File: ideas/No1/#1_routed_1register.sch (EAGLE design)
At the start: 17 parts, among them IC1 ULN2803, IC2 ULN2803, IC3 TD620831A, IC4 TD620831A, U1 SN74HC595N, U2 SN74HC595N, U3 SN74HC595N, U4 SN74HC595N

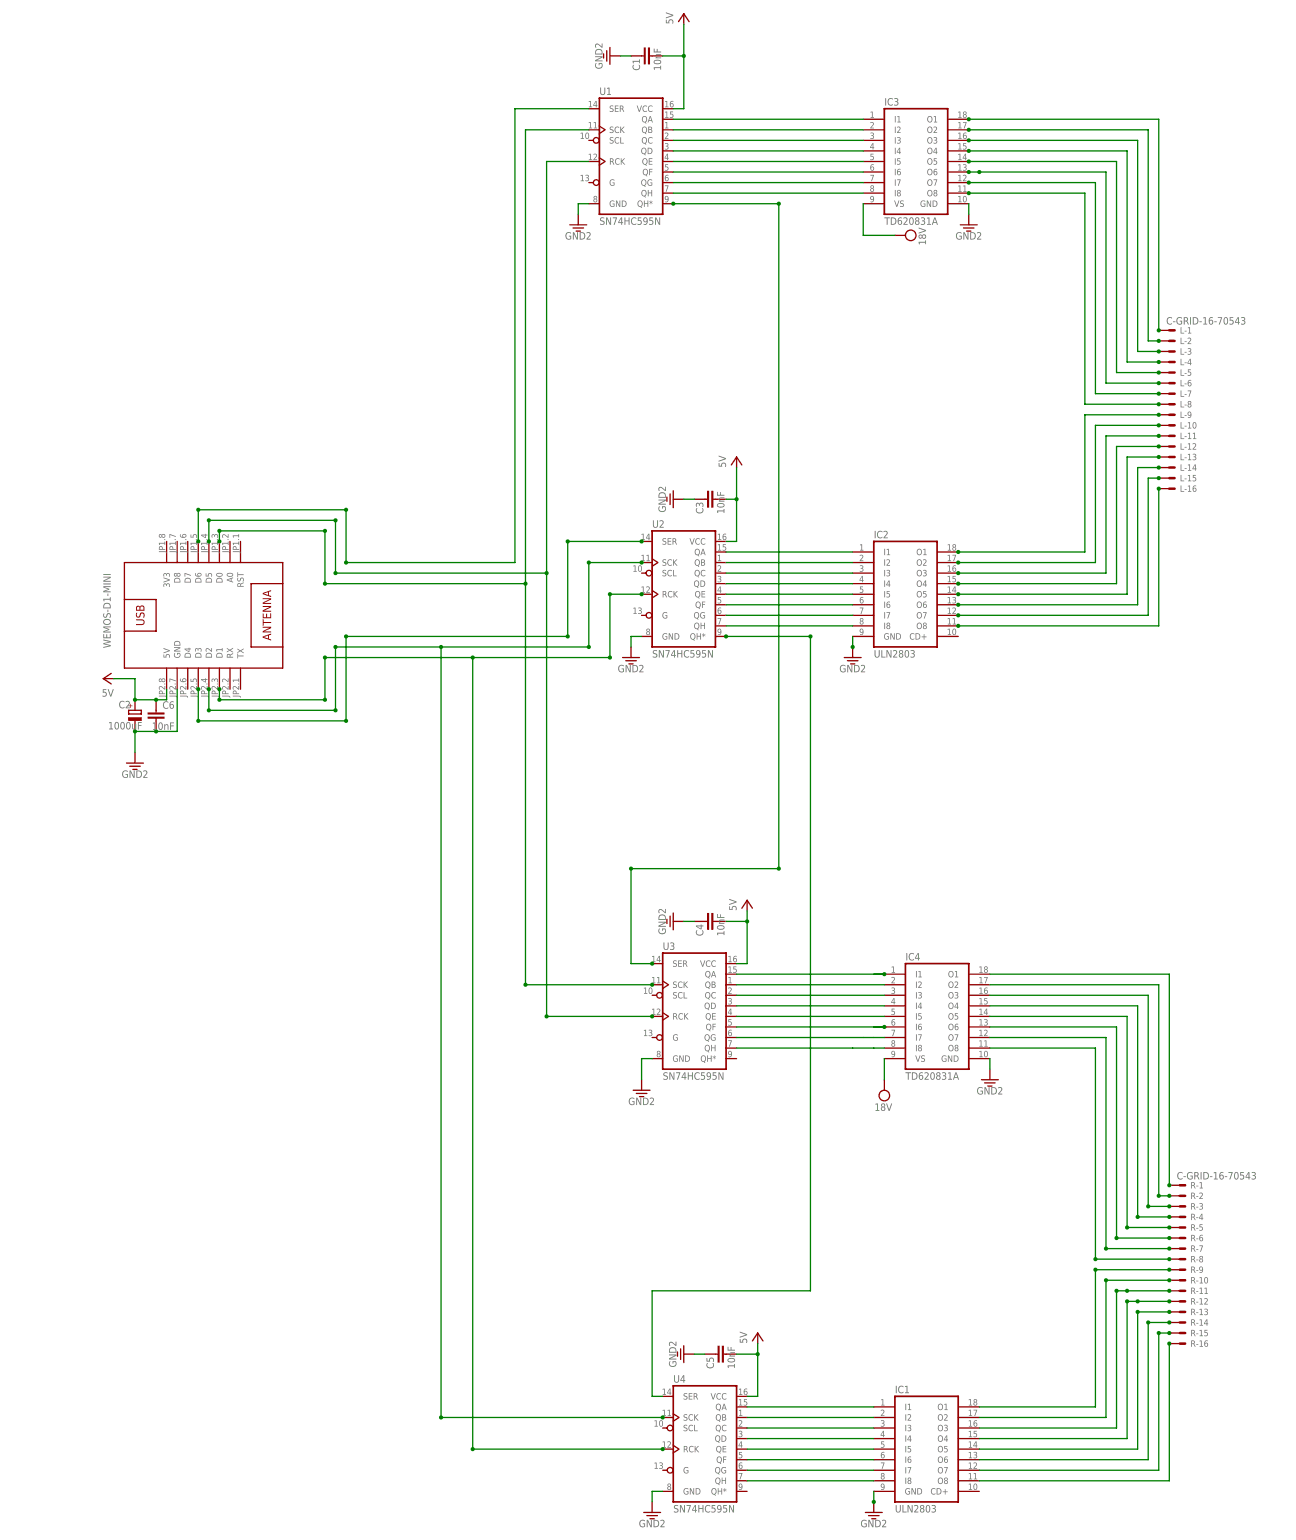
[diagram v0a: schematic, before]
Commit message: 1_route_1register.sch
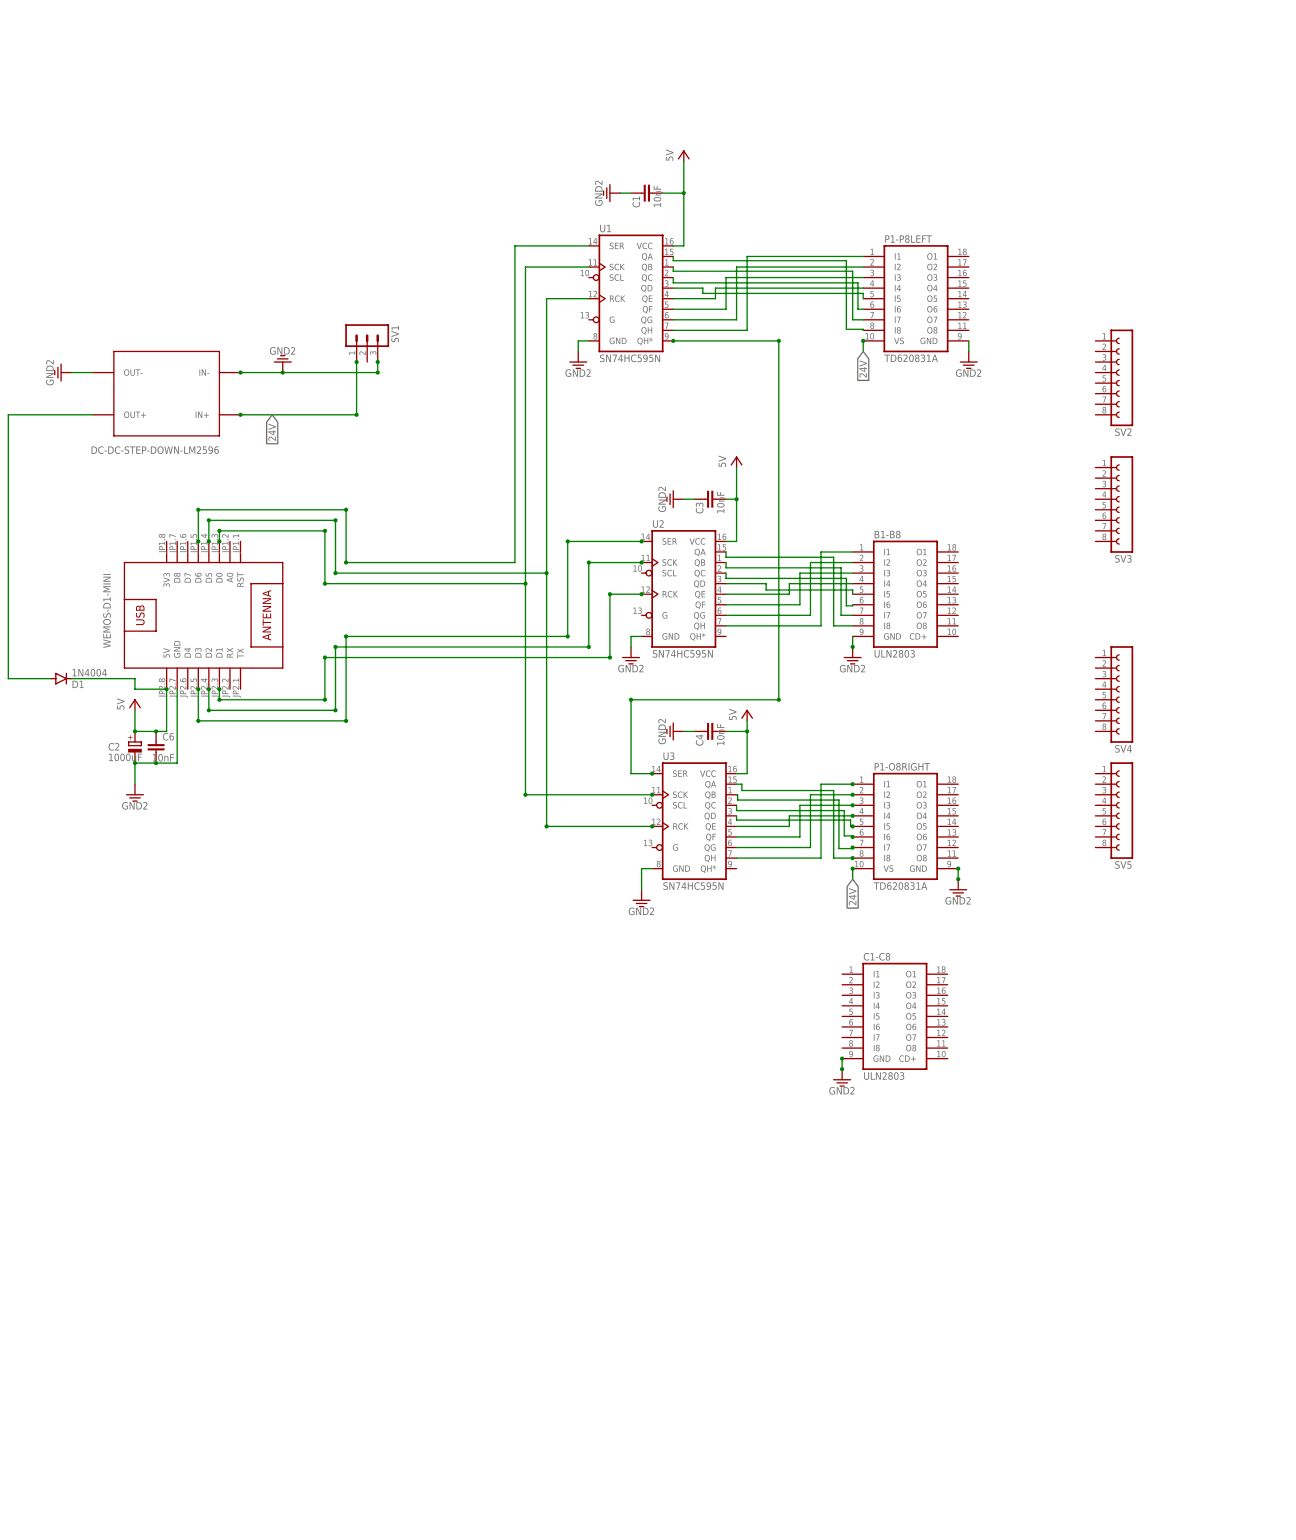
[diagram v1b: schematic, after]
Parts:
- removed C5: 10nF, resistor:C-EU025-025X050
- removed IC1: ULN2803, uln-udn:ULN2803A
- removed IC3, IC4: TD620831A, td62083-dil:TD620831A
- removed L, R: C-GRID-16-70543, con-molex:C-GRID-16-70543
- removed U4: SN74HC595N, SparkFun-IC-Logic:74HC595N
- added C1-C8: ULN2803, uln-udn:ULN2803A
- added D1: 1N4004, diode:1N4004
- added P1-O8RIGHT, P1-P8LEFT: TD620831A, td62083-dil:TD620831A
- added SV1: (no value), con-lstb:MA03-1
- added SV2, SV3, SV4, SV5: (no value), con-lsta:FE08-1
- added U$2: DC-DC-STEP-DOWN-LM2596, diy-modules_lm2596:DC-DC-STEP-DOWN-LM2596
- renumbered IC2 to B1-B8
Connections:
- removed net N$10: IC3.O2, L-2.S
- removed net N$11: IC3.O3, L-3.S
- removed net N$12: IC3.O4, L-4.S
- removed net N$13: IC3.O5, L-5.S
- removed net N$14: IC3.O6, L-6.S
- removed net N$15: IC3.O7, L-7.S
- removed net N$16: IC3.O8, L-8.S
- removed net N$17: B1-B8.O8, L-16.S
- removed net N$18: B1-B8.O7, L-15.S
- removed net N$19: B1-B8.O6, L-14.S
- removed net N$20: B1-B8.O5, L-13.S
- removed net N$21: B1-B8.O4, L-12.S
- removed net N$22: B1-B8.O3, L-11.S
- removed net N$23: B1-B8.O2, L-10.S
- removed net N$24: B1-B8.O1, L-9.S
- removed net N$26: IC4.O2, R-2.S
- removed net N$28: IC4.O4, R-4.S
- removed net N$30: IC4.O6, R-6.S
- removed net N$33: IC4.O8, R-8.S
- removed net N$35: IC4.I8, U3.QH
- removed net N$39: IC1.O8, R-16.S
- removed net N$40: IC1.O7, R-15.S
- removed net N$49: IC1.O6, R-14.S
- removed net N$50: IC1.O5, R-13.S
- removed net N$51: IC1.O4, R-12.S
- removed net N$52: IC1.O3, R-11.S
- removed net N$53: IC1.O2, R-10.S
- removed net N$54: IC1.O1, R-9.S
- removed net N$57: IC4.O1, R-1.S
- removed net N$59: IC4.O3, R-3.S
- removed net N$61: IC4.O5, R-5.S
- removed net N$63: IC4.O7, R-7.S
- removed net N$73: IC4.I2, U3.QB
- removed net N$74: IC4.I3, U3.QC
- removed net N$75: IC4.I4, U3.QD
- removed net N$76: IC4.I5, U3.QE
- removed net N$77: U2.QH*, U4.SER
- removed net N$78: IC4.I7, U3.QG
- removed net N$83: IC1.I1, U4.QA
- removed net N$84: IC1.I2, U4.QB
- removed net N$85: IC1.I3, U4.QC
- removed net N$86: IC1.I4, U4.QD
- removed net N$87: IC1.I5, U4.QE
- removed net N$88: IC1.I6, U4.QF
- removed net N$89: IC1.I7, U4.QG
- removed net N$9: IC3.O1, L-1.S
- removed net N$90: IC1.I8, U4.QH
- new net 24V: P1-O8RIGHT.VS, P1-P8LEFT.VS, SV1.1, U$2.IN+
- new net GND: B1-B8.GND, C1-C8.GND, C1.1, C2.-, C3.1, C4.1, C6.2, P1-O8RIGHT.GND, P1-P8LEFT.GND, U$1.GND, U1.GND, U2.GND, U3.GND
- new net N$25: P1-P8LEFT.I1, U1.QH
- new net N$27: P1-P8LEFT.I2, U1.QG
- new net N$29: P1-P8LEFT.I3, U1.QF
- new net N$32: P1-P8LEFT.I5, U1.QD
- new net N$55: P1-O8RIGHT.I7, U3.QB
- new net N$56: P1-O8RIGHT.I8, U3.QA
- new net N$69: D1.A, U$2.OUT+
- net 3.3V: now also SV1.3, U$2.IN-, U$2.OUT-; no longer B1-B8.GND, C1.1, C2.-, C3.1, C4.1, C5.1, C6.2, IC1.GND, IC3.GND, IC4.GND, U$1.GND, U1.GND, U2.GND, U3.GND, U4.GND
- net N$1: now also U2.QH; no longer U2.QA
- net N$2: now also U2.QG; no longer U2.QB
- net N$3: now also U2.QF; no longer U2.QC
- net N$31: now also P1-P8LEFT.I4, U1.QE; no longer IC3.I8, U1.QH
- net N$38: no longer U4.RCK
- net N$4: now also U2.QE; no longer U2.QD
- net N$41: now also P1-P8LEFT.I6, U1.QC; no longer IC3.I1, U1.QA
- net N$42: now also P1-P8LEFT.I7; no longer IC3.I2
- net N$43: now also P1-P8LEFT.I8, U1.QA; no longer IC3.I3, U1.QC
- net N$44: now also P1-O8RIGHT.I2, U3.QG; no longer IC3.I4, U1.QD
- net N$45: now also P1-O8RIGHT.I3, U3.QF; no longer IC3.I5, U1.QE
- net N$46: now also P1-O8RIGHT.I4, U3.QE; no longer IC4.I6, U3.QF
- net N$47: now also P1-O8RIGHT.I5, U3.QD; no longer IC3.I7, U1.QG
- net N$48: now also P1-O8RIGHT.I6, U3.QC; no longer IC3.I6, U1.QF
- net N$5: now also U2.QD; no longer U2.QE
- net N$6: now also U2.QC; no longer U2.QF
- net N$7: now also U2.QB; no longer U2.QG
- net N$72: now also P1-O8RIGHT.I1, U3.QH; no longer IC4.I1, U3.QA
- net N$8: now also U2.QA; no longer U2.QH
- net N$80: no longer U4.SCK
- net VCC: now also D1.C; no longer C5.2, IC3.VS, IC4.VS, U4.VCC
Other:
- moved on the sheet: C1, C2, C4, C6, U1, U3
